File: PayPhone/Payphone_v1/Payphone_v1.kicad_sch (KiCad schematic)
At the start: 4 parts, among them J1 JST_05, K1 G6S-2, U1 MCP23008-xP, U2 MC34063AP

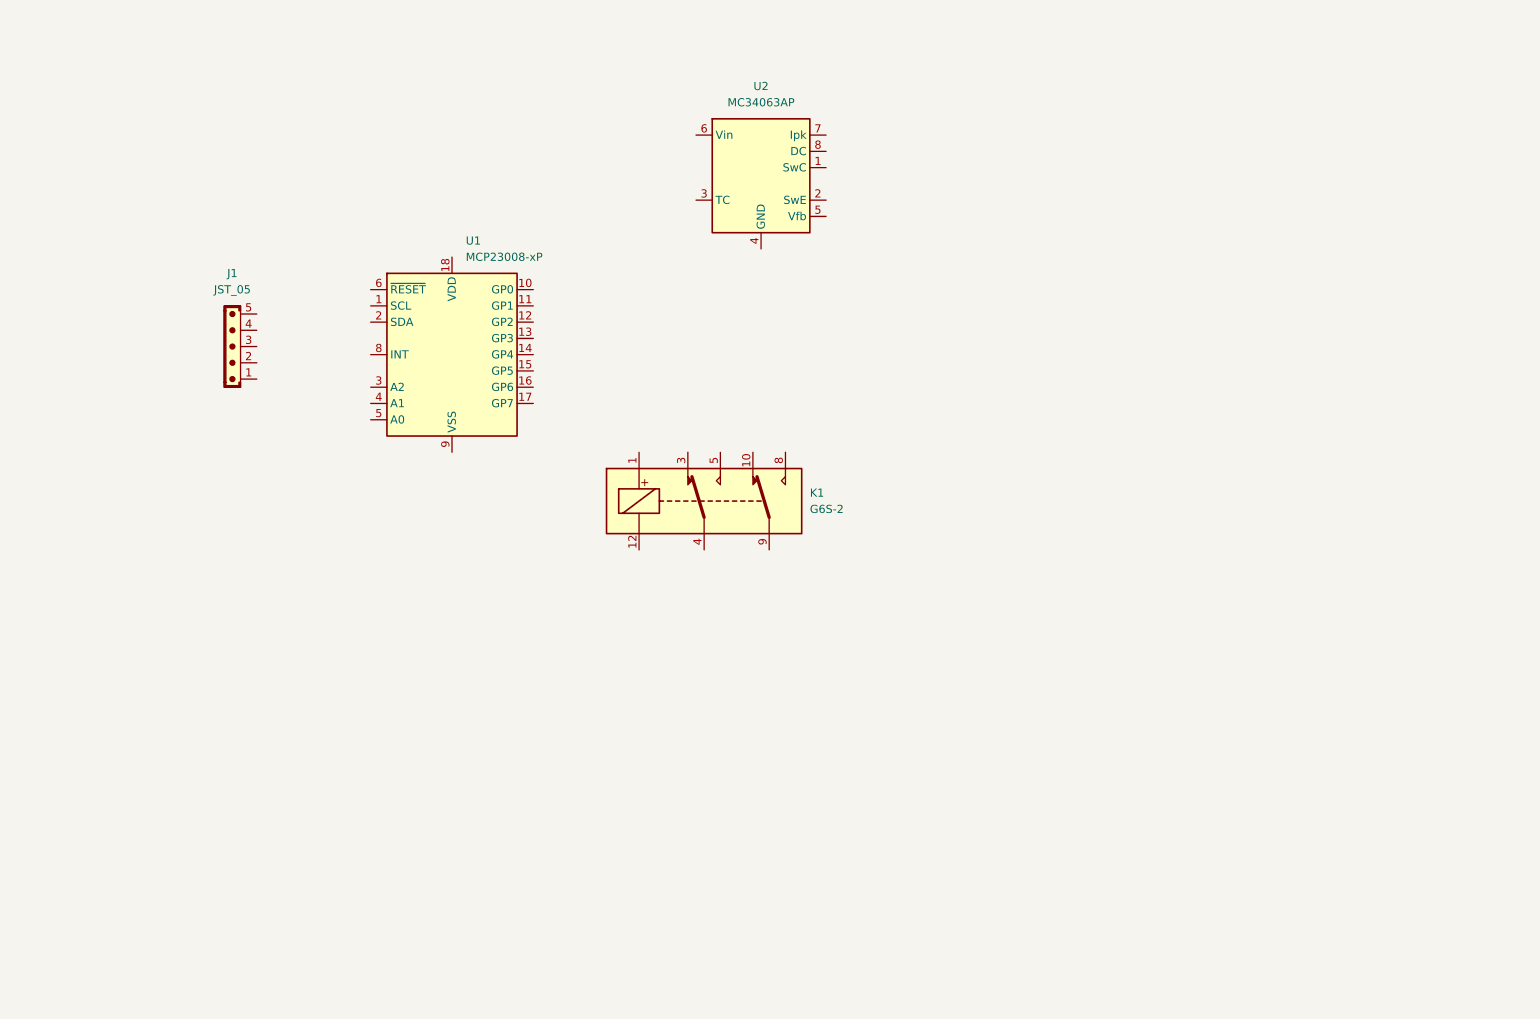
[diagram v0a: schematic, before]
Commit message: Payphone_v1: all active parts, diodes, C_out, inductors, trimmer and connectors placed with footprints (no wires)
Co-Authored-By: Claude Sonnet 5.5 <noreply@anthropic.com>
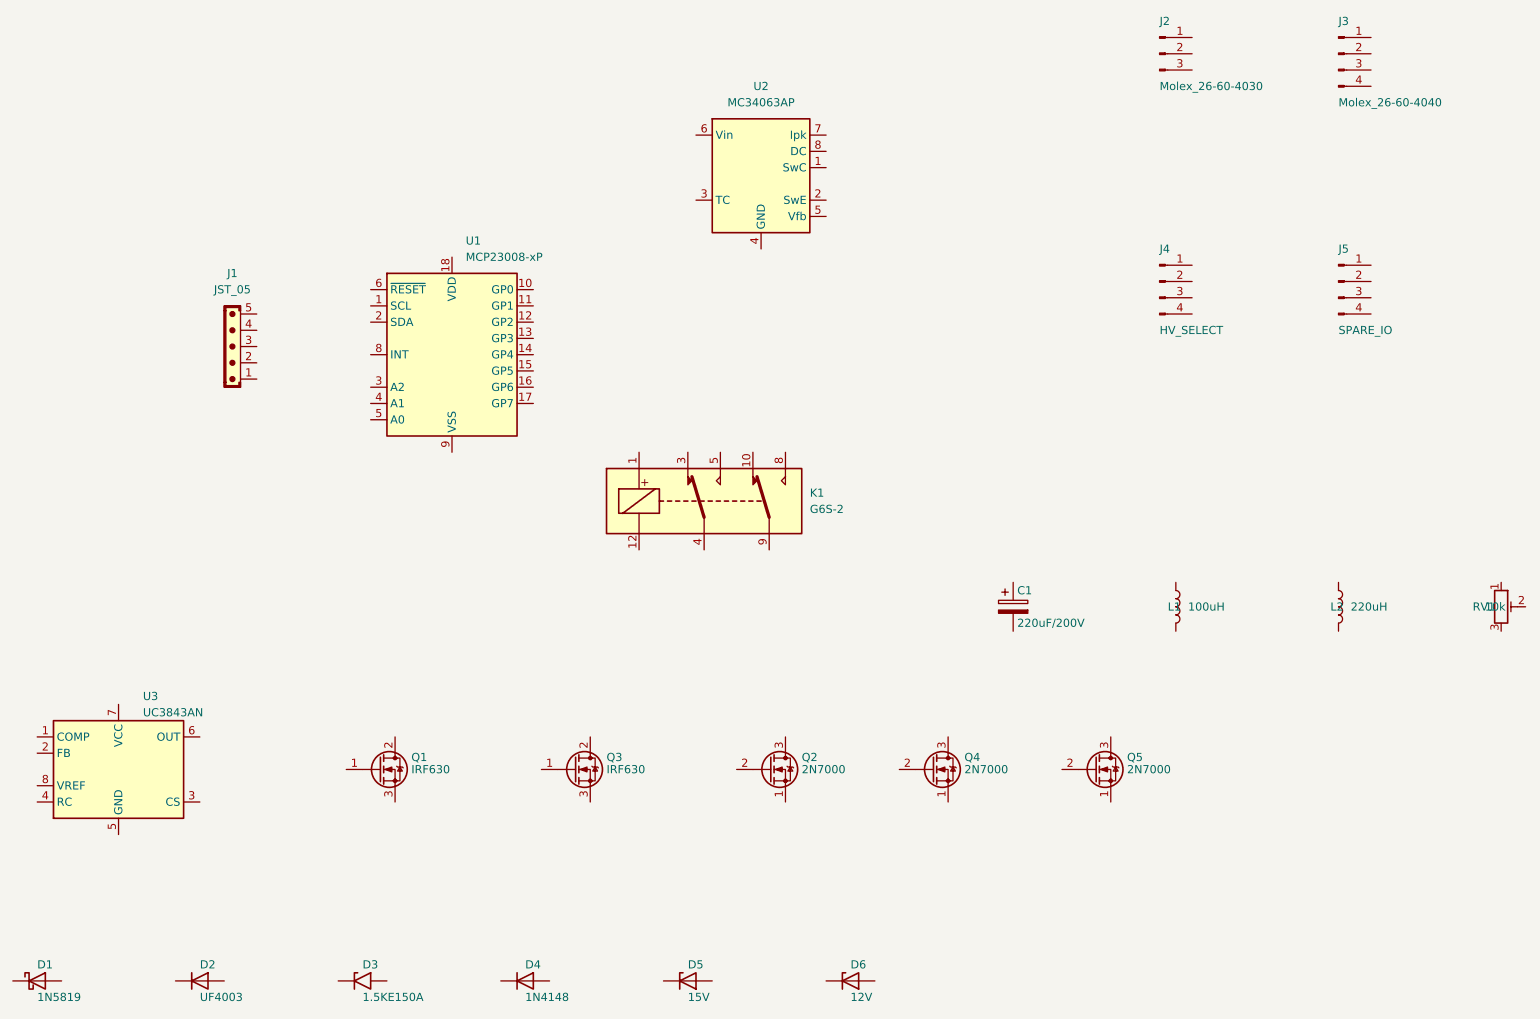
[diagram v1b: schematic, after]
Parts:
- added C1: 220uF/200V, Capacitor_THT:CP_Radial_D18.0mm_P7.50mm, symbol Device:C_Polarized
- added D1: 1N5819, Diode_THT:D_DO-41_SOD81_P10.16mm_Horizontal, symbol Diode:1N5819
- added D2: UF4003, Diode_THT:D_DO-41_SOD81_P10.16mm_Horizontal, symbol Custom:UF4003
- added D3: 1.5KE150A, Diode_THT:D_DO-201AD_P15.24mm_Horizontal, symbol Diode:1.5KExxA
- added D4: 1N4148, Diode_THT:D_DO-35_SOD27_P7.62mm_Horizontal, symbol Diode:1N4148
- added D5: 15V, Diode_THT:D_DO-41_SOD81_P10.16mm_Horizontal, symbol Device:D_Zener
- added D6: 12V, Diode_THT:D_DO-41_SOD81_P10.16mm_Horizontal, symbol Device:D_Zener
- added J2: Molex_26-60-4030, Connector_Molex:Molex_KK-396_A-41791-0003_1x03_P3.96mm_Vertical, symbol Connector:Conn_01x03_Pin
- added J3: Molex_26-60-4040, Connector_Molex:Molex_KK-396_A-41791-0004_1x04_P3.96mm_Vertical, symbol Connector:Conn_01x04_Pin
- added J4: HV_SELECT, Connector_PinHeader_2.54mm:PinHeader_1x04_P2.54mm_Vertical, symbol Connector:Conn_01x04_Pin
- added J5: SPARE_IO, Connector_PinHeader_2.54mm:PinHeader_1x04_P2.54mm_Vertical, symbol Connector:Conn_01x04_Pin
- added L1: 100uH, Inductor_THT:L_Radial_D10.0mm_P5.00mm_Fastron_07M, symbol Device:L
- added L2: 220uH, Inductor_THT:L_Radial_D10.0mm_P5.00mm_Fastron_07M, symbol Device:L
- added Q1, Q3: IRF630, Package_TO_SOT_THT:TO-220-3_Vertical, symbol Custom:IRF630
- added Q2, Q4, Q5: 2N7000, Package_TO_SOT_THT:TO-92_Inline, symbol Transistor_FET:2N7000
- added RV1: 10k, Potentiometer_THT:Potentiometer_Bourns_3296W_Vertical, symbol Device:R_Potentiometer_Trim
- added U3: UC3843AN, Package_DIP:DIP-8_W7.62mm, symbol Custom:UC3843AN
